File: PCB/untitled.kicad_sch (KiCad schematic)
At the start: 1 part, among them U2 MPU-6050

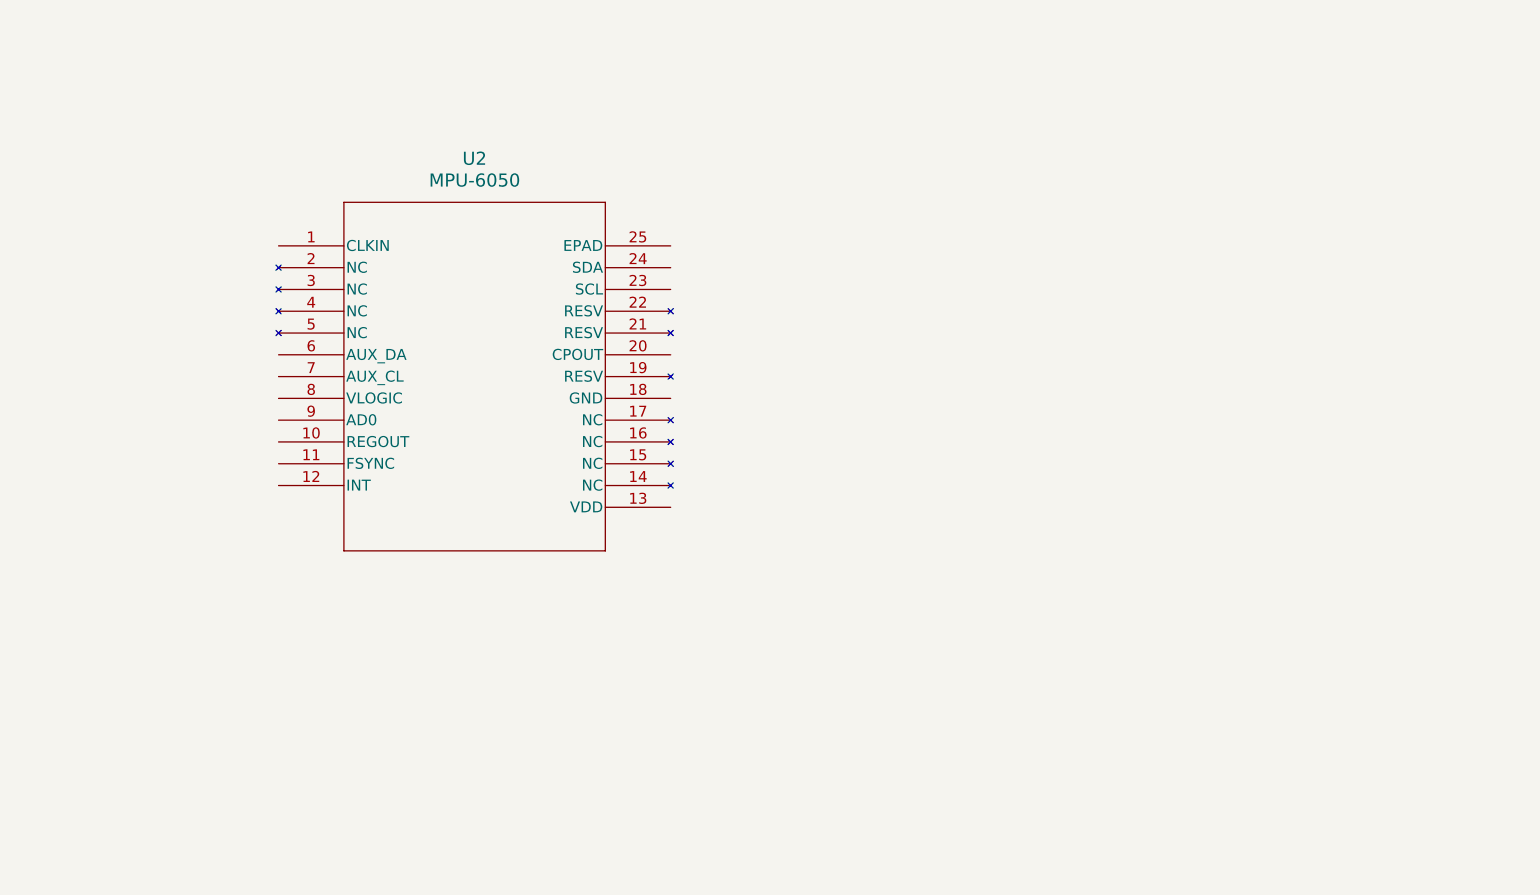
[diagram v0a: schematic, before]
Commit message: work on IMU
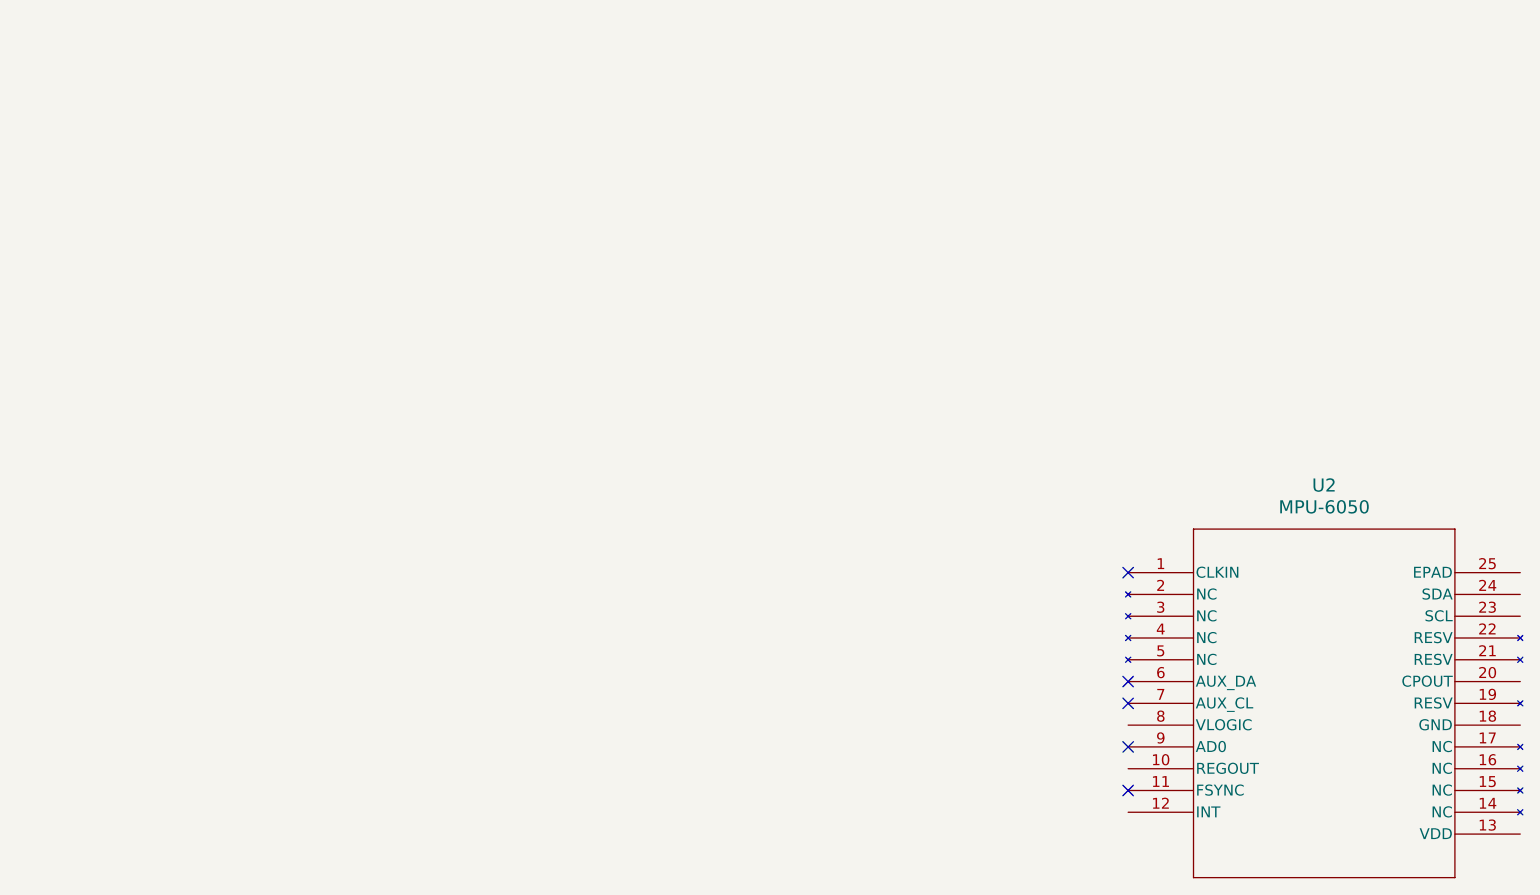
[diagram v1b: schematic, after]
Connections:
- no-connect marks 0 -> 5
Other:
- moved on the sheet: U2
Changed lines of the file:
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@@
 	(generator_version "9.0")
 	(paper "A4")
+	(no_connect
+		(at 143.51 78.74)
+	)
+	(no_connect
+		(at 143.51 93.98)
+	)
+	(no_connect
+		(at 143.51 104.14)
+	)
+	(no_connect
+		(at 143.51 91.44)
+	)
+	(no_connect
+		(at 143.51 99.06)
+	)
 	(symbol
 		(lib_id "IMU:MPU-6050")
-		(at 44.45 40.64 0)
+		(at 143.51 78.74 0)
 		(unit 1)
 		(exclude_from_sim no)
@@
 		(fields_autoplaced yes)
 		(property "Reference" "U2"
-			(at 67.31 30.48 0)
+			(at 166.37 68.58 0)
 			(effects
 				(font
@@
 		)
 		(property "Value" "MPU-6050"
-			(at 67.31 33.02 0)
+			(at 166.37 71.12 0)
 			(effects
 				(font
@@
 		)
 		(property "Footprint" "IMU:QFN24_4X4X0P9-0P5_TDK-L"
-			(at 44.45 40.64 0)
+			(at 143.51 78.74 0)
 			(effects
 				(font
@@
 		)
 		(property "Datasheet" "MPU-6050"
-			(at 44.45 40.64 0)
+			(at 143.51 78.74 0)
 			(effects
 				(font
@@
 		)
 		(property "Description" ""
-			(at 44.45 40.64 0)
+			(at 143.51 78.74 0)
 			(effects
 				(font

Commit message: IMU done yay
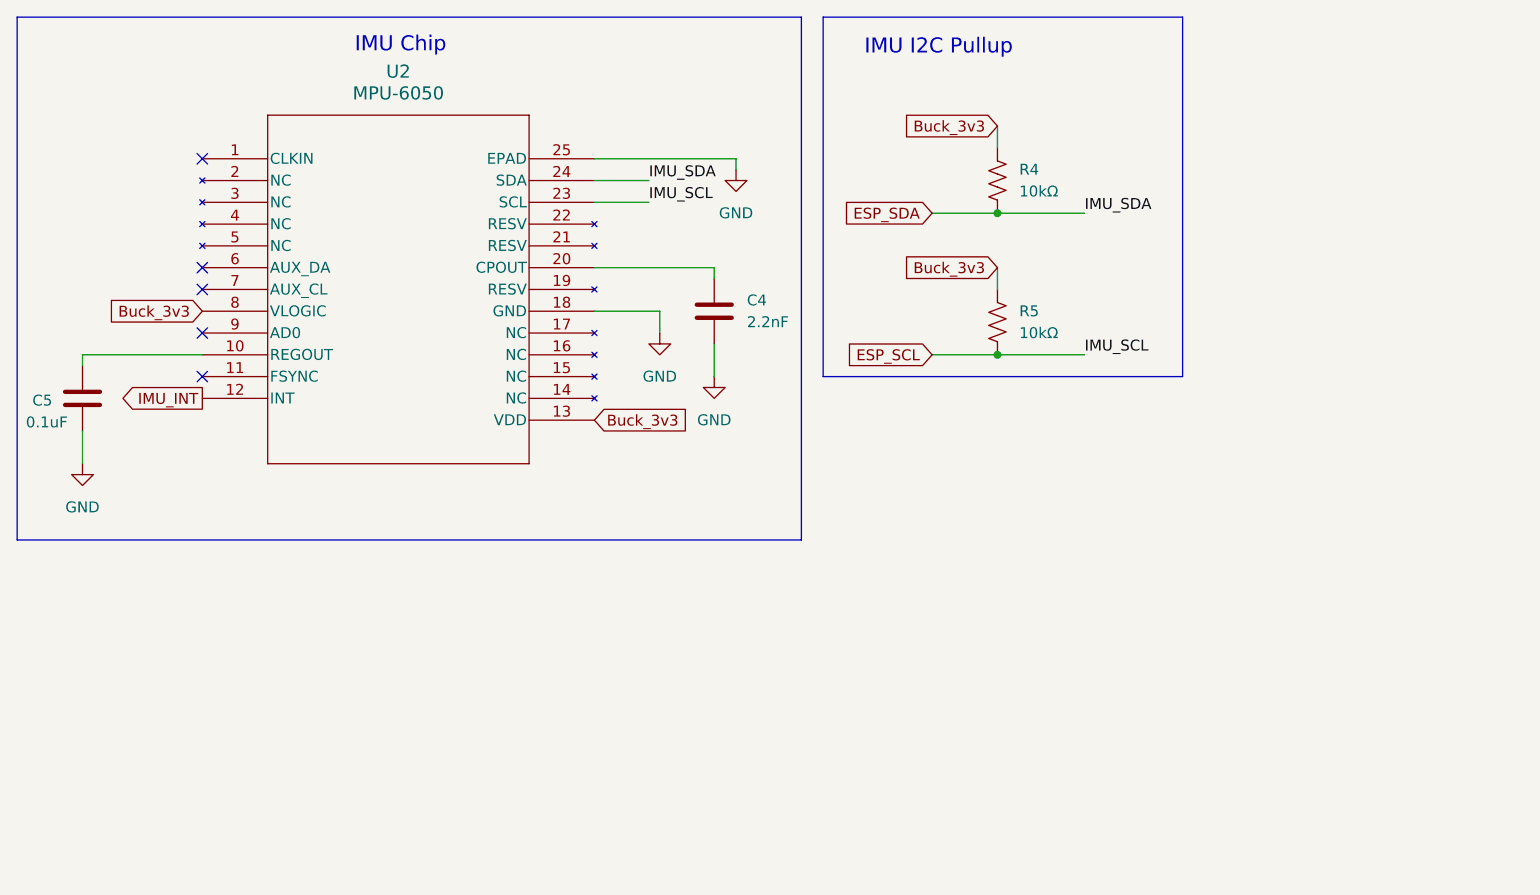
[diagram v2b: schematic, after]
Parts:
- added C4: 2.2nF, symbol Device:C
- added C5: 0.1uF, symbol Device:C
- added R4, R5: 10kΩ, symbol Device:R_US
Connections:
- net at U2.10 (REGOUT): now also C5.1
- net IMU_INT: now reaches U2.12 (INT)
- net Buck_3v3: now reaches U2.13 (VDD)
- net Buck_3v3: now also U2.8 (VLOGIC), R4.1, R5.1
- net GND: now reaches U2.18 (GND)
- net GND: now also U2.25 (EPAD), C4.2, C5.2
- net at U2.20 (CPOUT): now also C4.1
- net ESP_SCL: now reaches U2.23 (SCL)
- net ESP_SCL: now also R5.2
- net ESP_SDA: now reaches U2.24 (SDA)
- net ESP_SDA: now also R4.2
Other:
- note added: "IMU Chip"
- note added: "IMU I2C Pullup"
- moved on the sheet: U2
